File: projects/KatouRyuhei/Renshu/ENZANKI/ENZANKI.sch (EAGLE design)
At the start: 25 parts

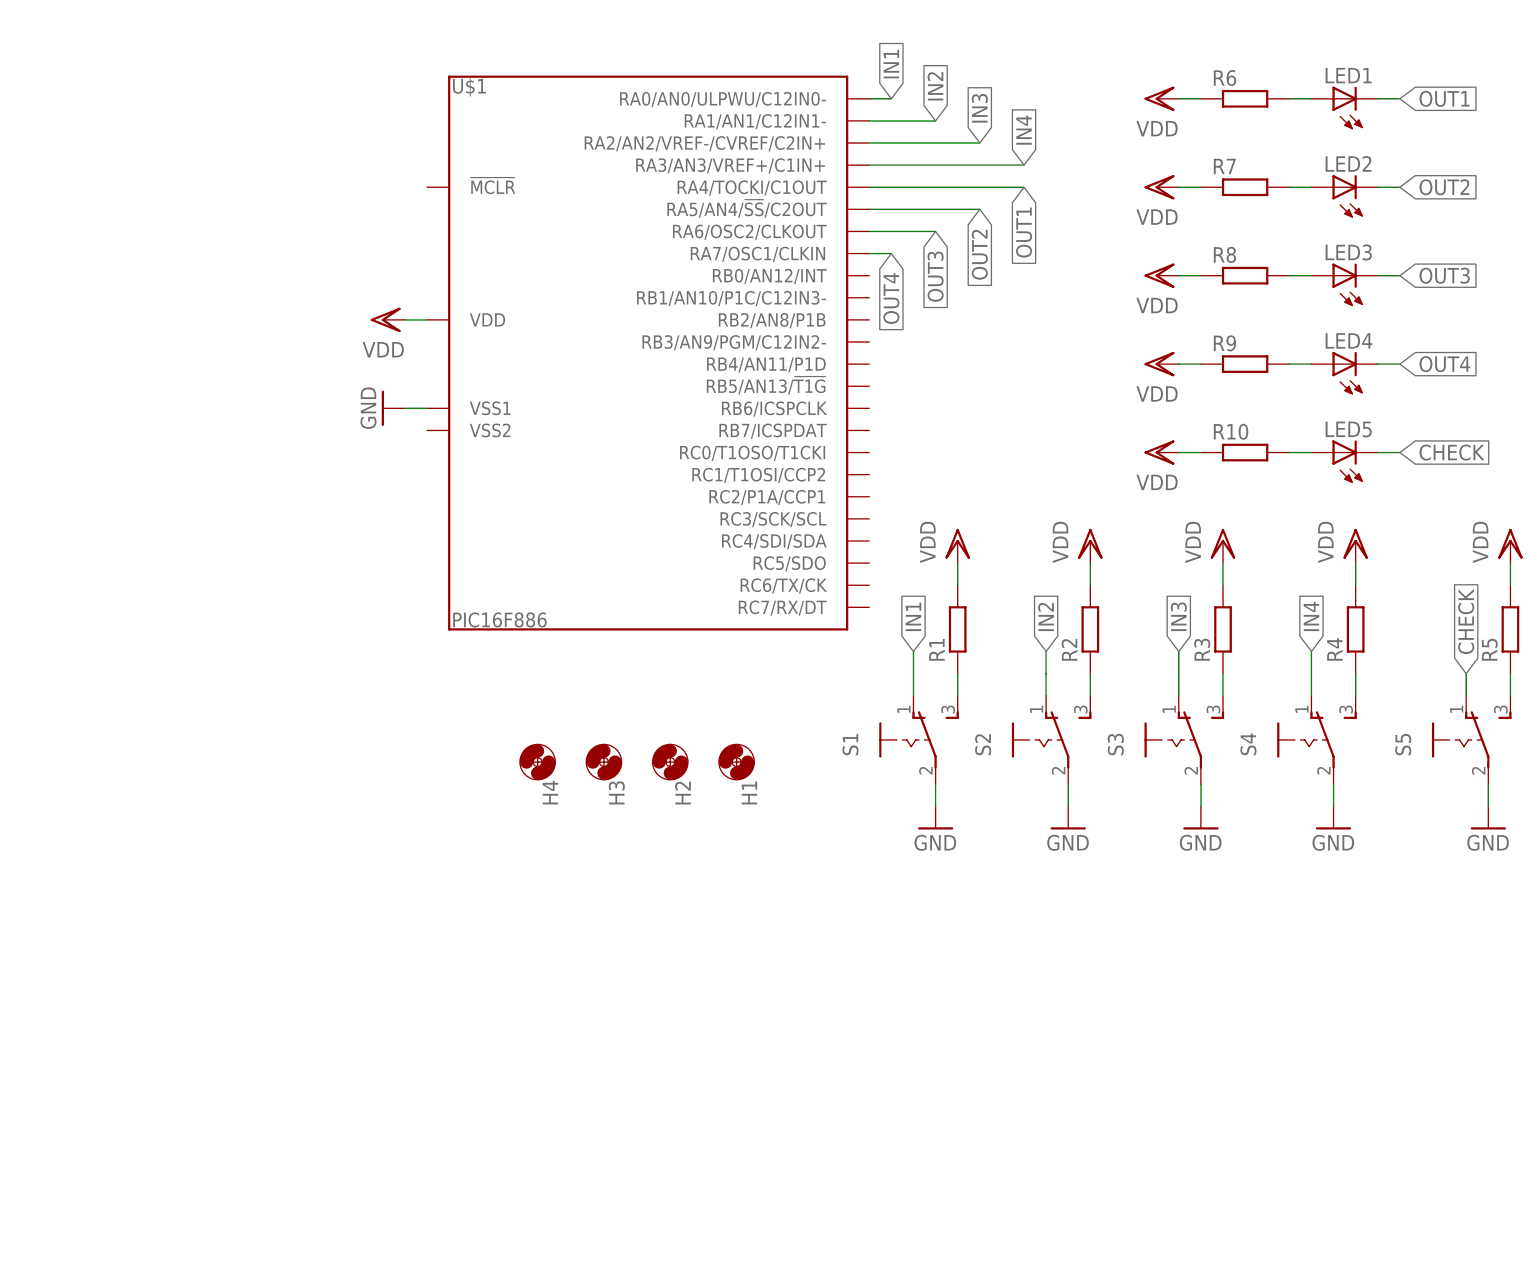
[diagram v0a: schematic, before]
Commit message: 回路図の作成
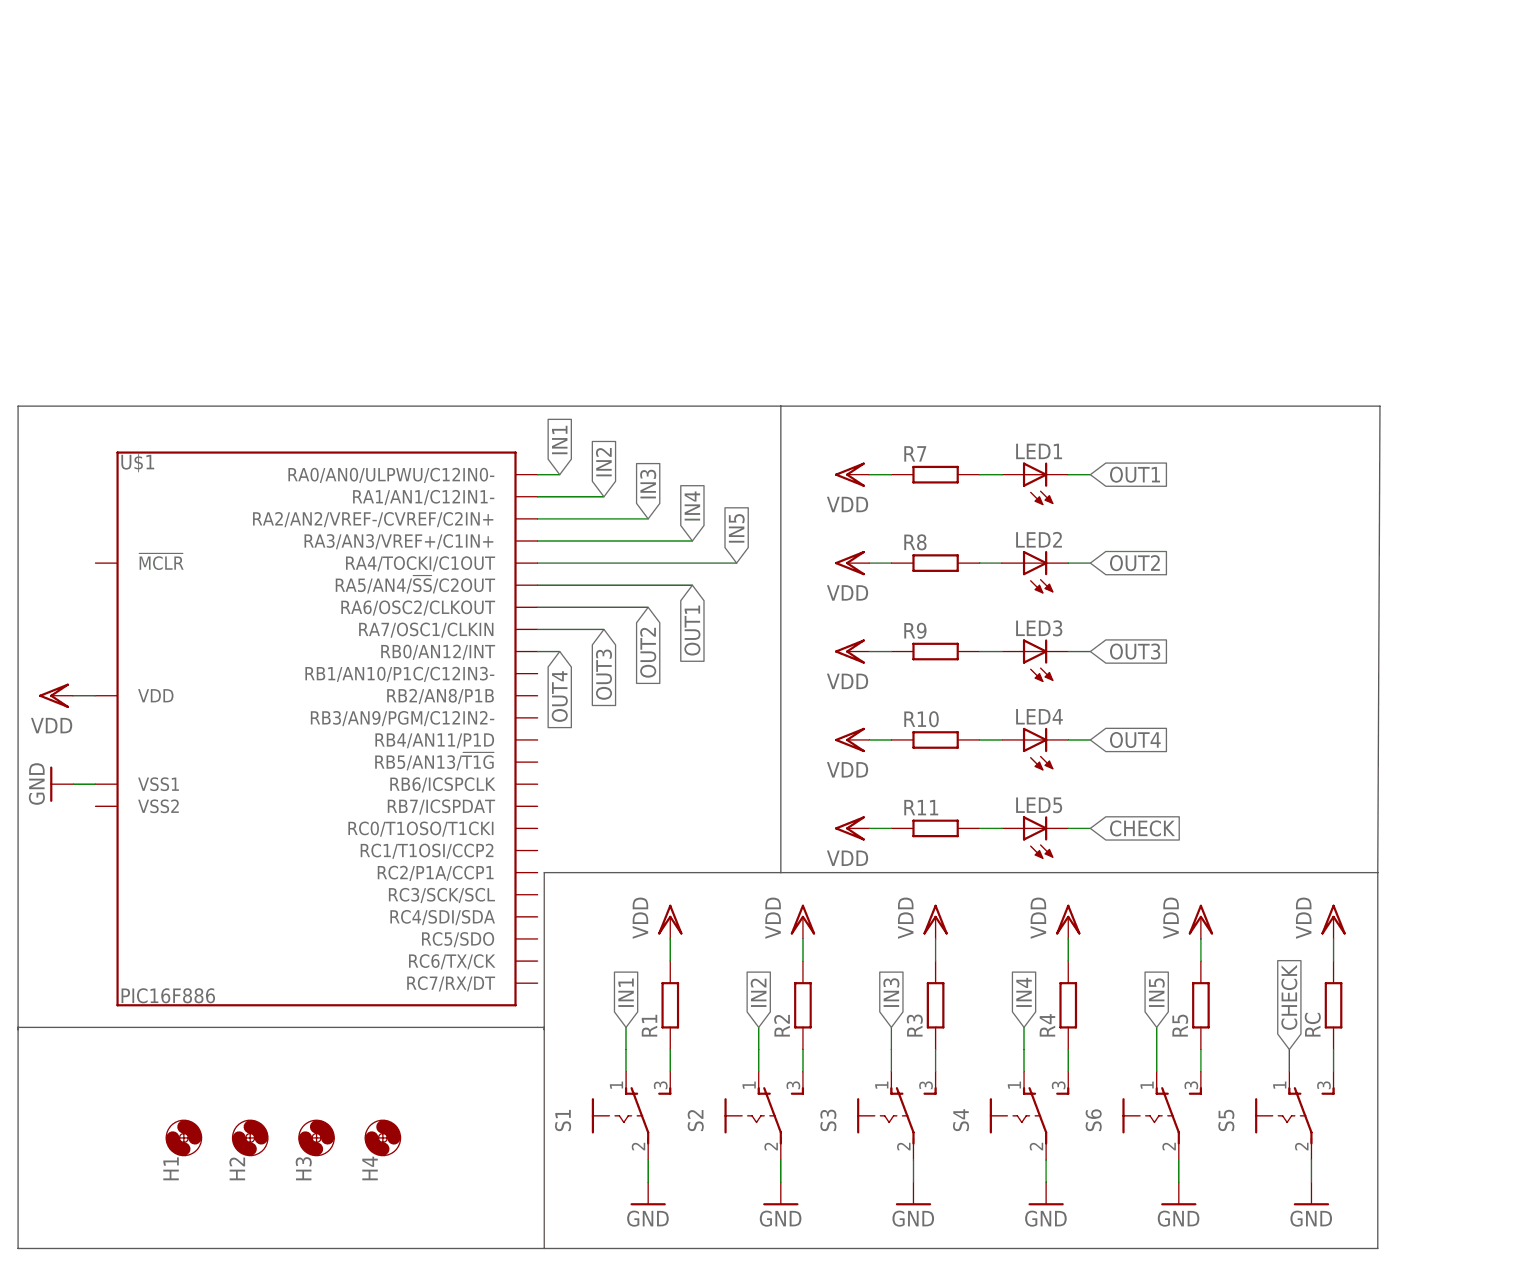
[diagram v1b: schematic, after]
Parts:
- removed R6: (no value), rcl:R-EU_R3216W
- added R11, RC: (no value), rcl:R-EU_R3216W
- added S6: (no value), switch:SLIDESW
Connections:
- new net IN5: S6.1, U$1.RA4/TOCKI/C1OUT
- new net N$10: R5.1, S6.3
- net GND: now also S6.2
- net N$1: now also R7.2; no longer R6.2
- net N$2: now also R8.2; no longer R7.2
- net N$3: now also R9.2; no longer R8.2
- net N$4: now also R10.2; no longer R9.2
- net N$5: now also RC.1; no longer R5.1
- net N$9: now also R11.2; no longer R10.2
- net OUT1: now also U$1.RA5/AN4/!SS!/C2OUT; no longer U$1.RA4/TOCKI/C1OUT
- net OUT2: now also U$1.RA6/OSC2/CLKOUT; no longer U$1.RA5/AN4/!SS!/C2OUT
- net OUT3: now also U$1.RA7/OSC1/CLKIN; no longer U$1.RA6/OSC2/CLKOUT
- net OUT4: now also U$1.RB0/AN12/INT; no longer U$1.RA7/OSC1/CLKIN
- net VDD: now also R11.1, RC.2; no longer R6.1
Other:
- moved on the sheet: H1, H2, H3, H4, LED1, LED2, LED3, LED4, LED5, R1, R10, R2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
